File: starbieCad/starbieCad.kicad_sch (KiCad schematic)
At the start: 5 parts, among them J1 MPU6050, SW1 SW_Push, SW2 SW_Push, U1 XIAO-ESP32-C3-SMD, U2 ER_OLEDM0.91_1x-I2C

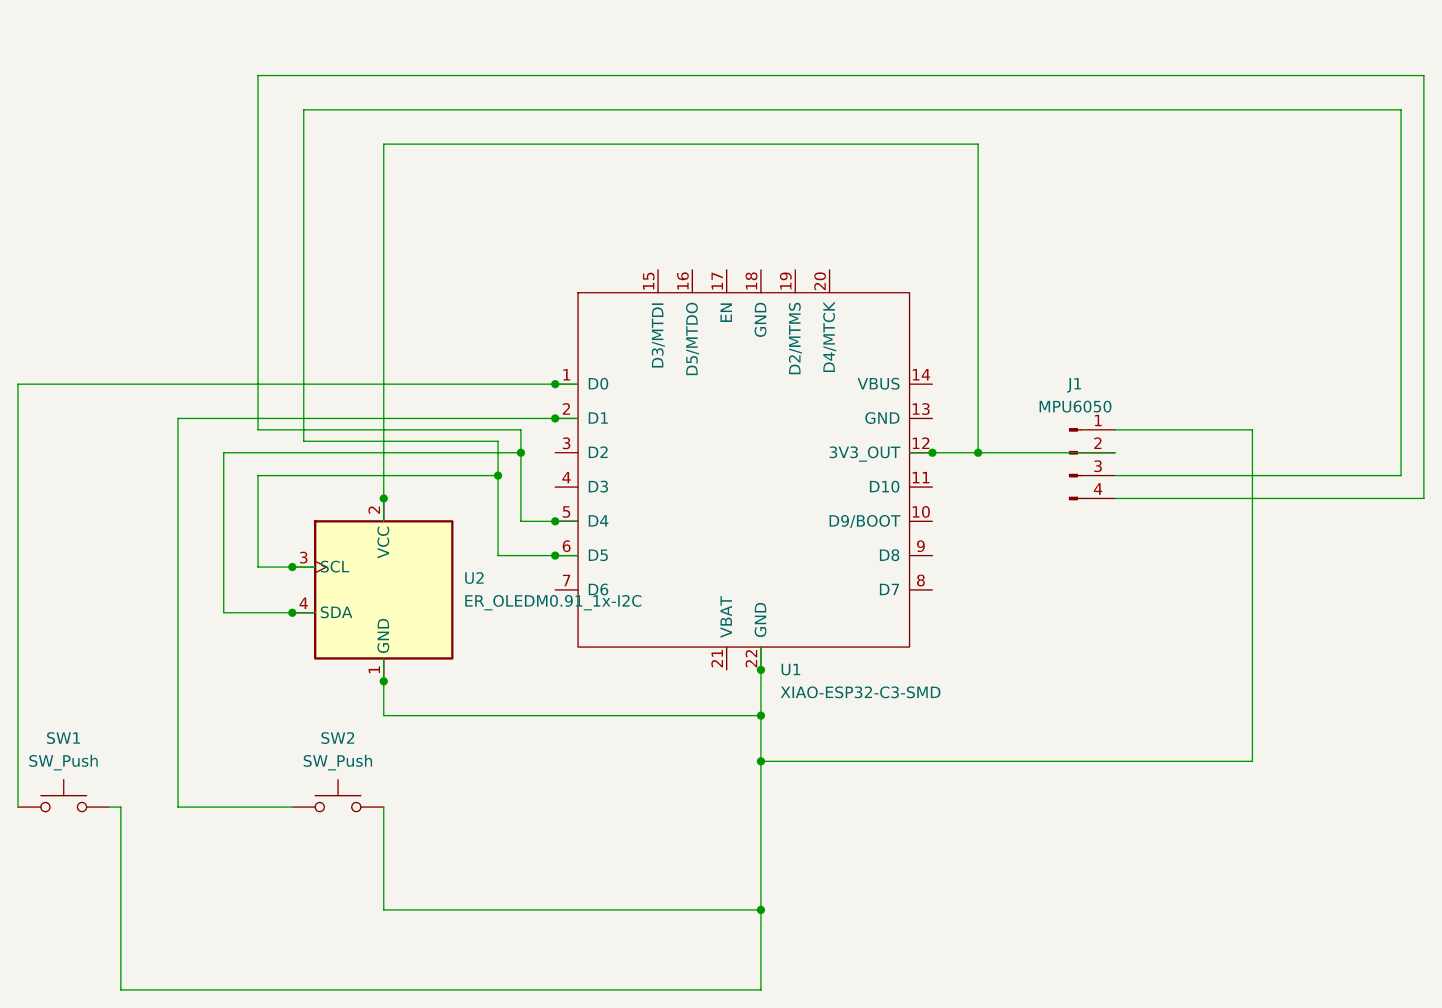
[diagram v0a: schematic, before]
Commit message: I finished all my shematics and pcb design and did all the circuit as well as the shape of the starbie
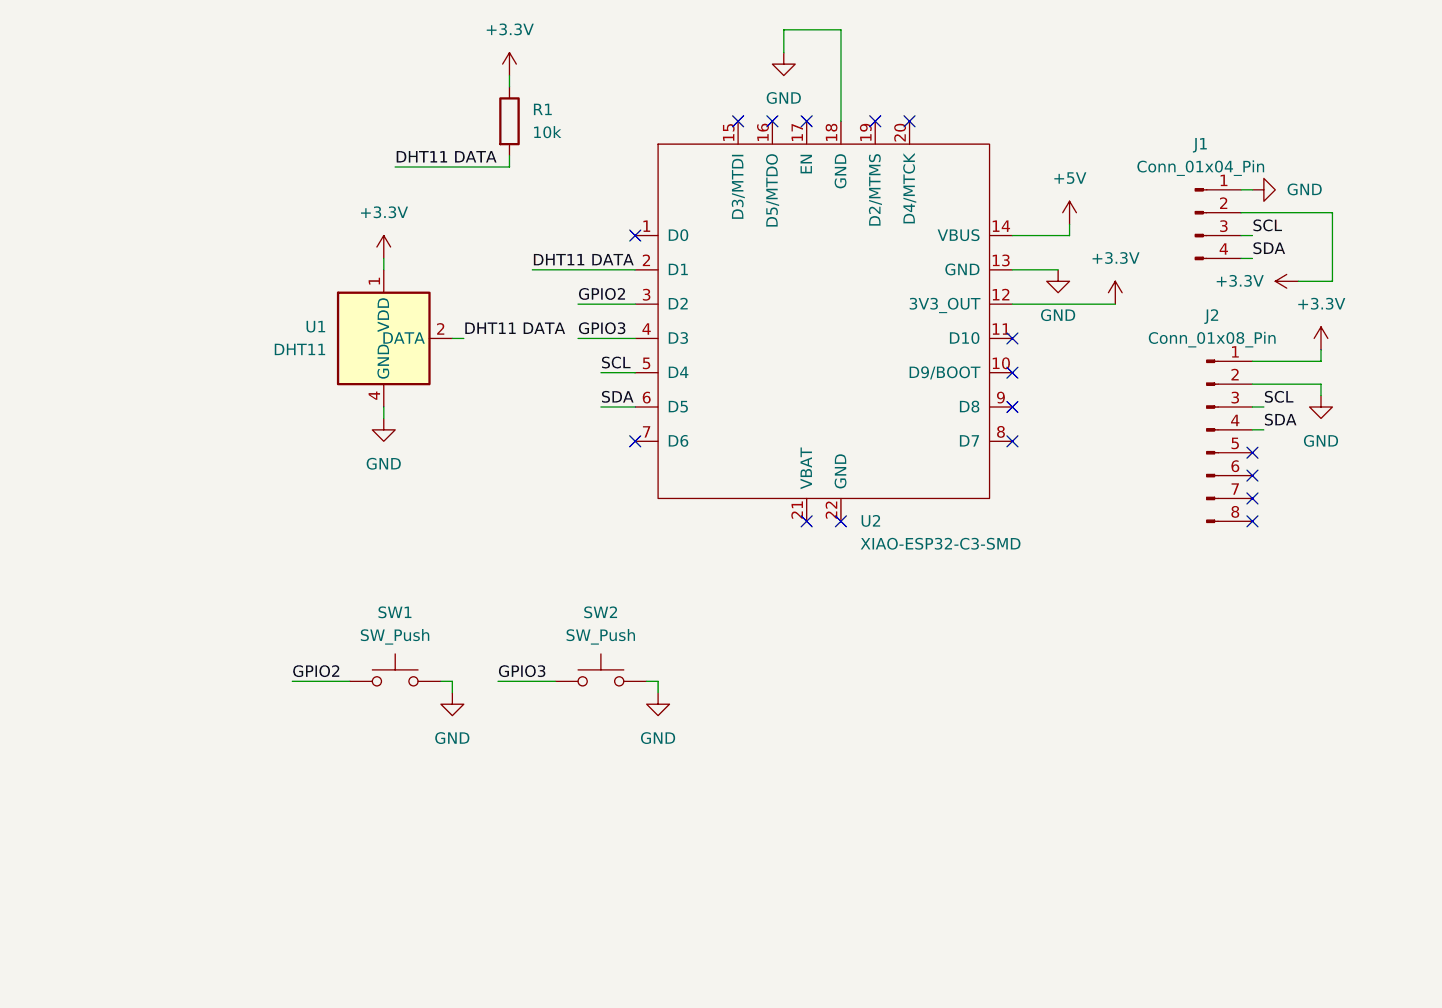
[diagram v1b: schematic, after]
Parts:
- removed U1: XIAO-ESP32-C3-SMD, Imported_Parts:XIAO-ESP32-C3-SMD, symbol Seeed_Studio_XIAO_Series:XIAO-ESP32-C3-SMD
- removed U2: ER_OLEDM0.91_1x-I2C, Connector_PinHeader_2.54mm:PinHeader_1x04_P2.54mm_Vertical, symbol Display_Graphic:ER_OLEDM0.91_1x-I2C
- added J2: Conn_01x08_Pin, Connector_PinHeader_2.54mm:PinHeader_1x08_P2.54mm_Vertical, symbol Connector:Conn_01x08_Pin
- added R1: 10k, Resistor_THT:R_Axial_DIN0204_L3.6mm_D1.6mm_P7.62mm_Horizontal, symbol Device:R
- added U1: DHT11, Sensor:Aosong_DHT11_5.5x12.0_P2.54mm, symbol Sensor:DHT11
- added U2: XIAO-ESP32-C3-SMD, Imported_Parts:XIAO-ESP32-C3-SMD, symbol Seeed_Studio_XIAO_Series:XIAO-ESP32-C3-SMD
- J1: value MPU6050 -> Conn_01x04_Pin; footprint Connector_PinHeader_2.54mm:PinHeader_1x04_P2.54mm_Vertical -> Imported_Parts:Display_128x64_096_I2C
- SW1, SW2: footprint Button_Switch_Keyboard:SW_Cherry_MX_1.00u_Plate -> Button_Switch_Keyboard:SW_Cherry_MX_1.00u_PCB
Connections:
- net GPIO3: now reaches SW2.1
- net GPIO3: now also U2.4 (D3)
- net GND: now reaches J1.1 (Pin_1), SW1.2, SW2.2
- net GND: now also J2.2 (Pin_2), U1.4 (GND), U2.13 (GND), U2.18 (GND)
- net +3.3V: now reaches J1.2 (Pin_2)
- net +3.3V: now also J2.1 (Pin_1), R1.1, U1.1 (VDD), U2.12 (3V3_OUT)
- net SCL: now reaches J1.3 (Pin_3)
- net SCL: now also J2.3 (Pin_3), U2.5 (D4)
- net SDA: now reaches J1.4 (Pin_4)
- net SDA: now also J2.4 (Pin_4), U2.6 (D5)
- net GPIO2: now reaches SW1.1
- net GPIO2: now also U2.3 (D2)
- new net +5V: U2.14 (VBUS)
- new net DHT11 DATA: R1.2, U1.2 (DATA), U2.2 (D1)
- no-connect marks 0 -> 17
